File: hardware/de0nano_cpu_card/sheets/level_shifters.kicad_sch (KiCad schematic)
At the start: 10 parts, among them J2 EXP_HEADER_2x11, U1 SN74LVC8T245, U2 SN74LVC8T245, U3 SN74LVC8T245, U4 SN74LVC8T245, U5 SN74LVC8T245, U6 SN74LVC8T245

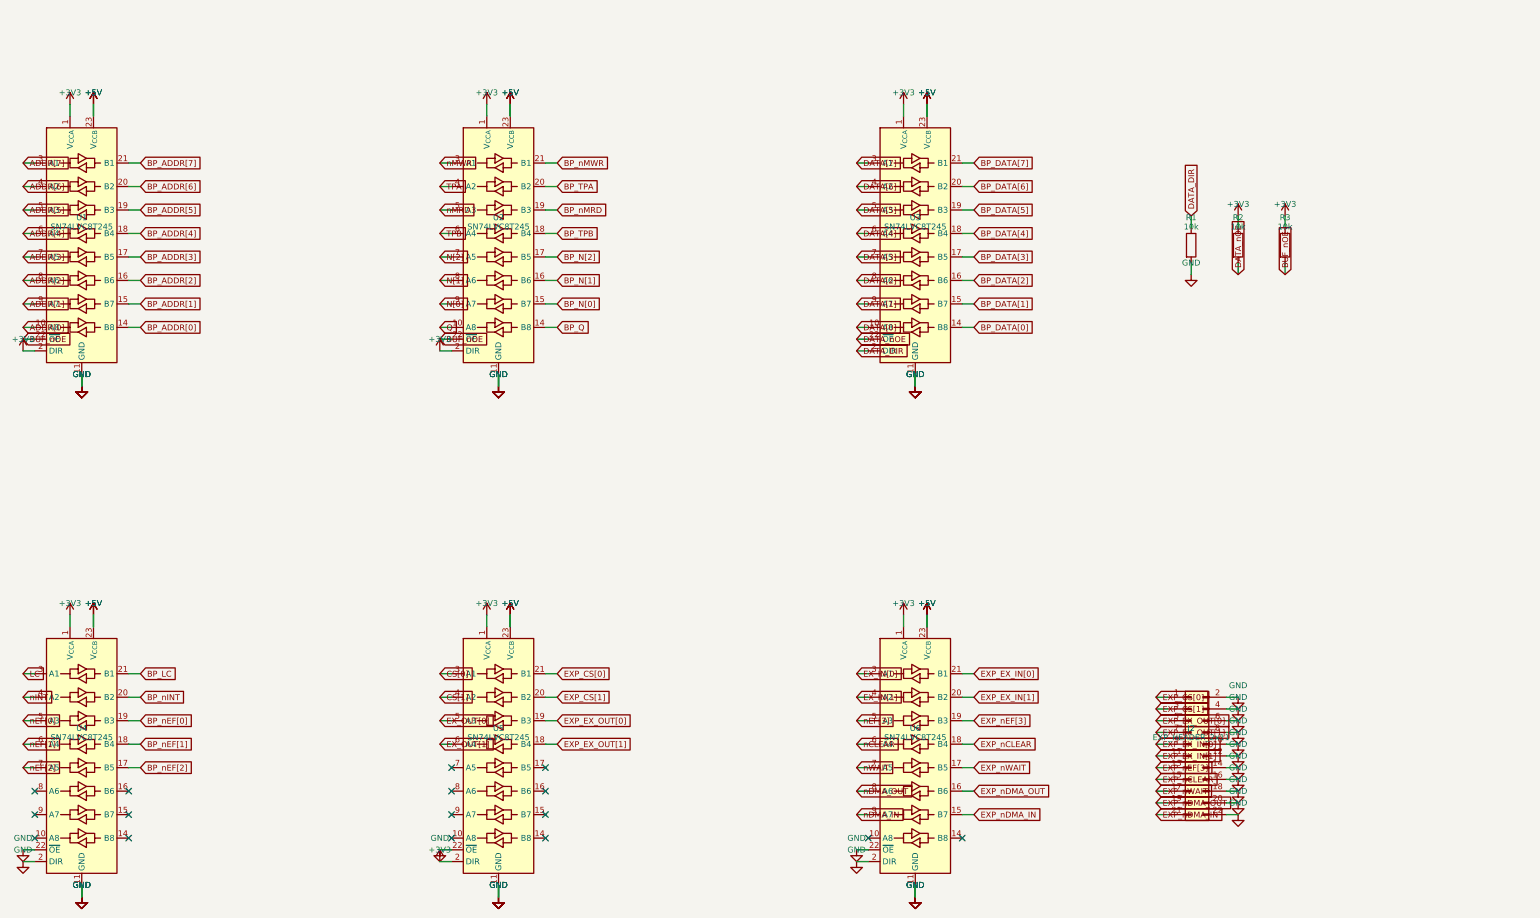
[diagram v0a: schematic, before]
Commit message: Add pull-ups/ties on spare channels and series resistors, per GUI review
The user reviewed the schematics in the KiCad GUI and manually
rearranged component layout on several sheets -- so these fixes are
applied as surgical patches to the current saved files (new
tools/patch_*.py scripts) rather than via the usual build_*.py
regeneration, which would have discarded that layout work. See the new
"don't just re-run build_*.py" section in tools/README.md for the
workflow this establishes going forward.

Electrical changes (level_shifters.kicad_sch):
- 10k pull-up to +5V on all 7 EXP_* future-expansion header input nets
- U4 (backplane IN chip) spare B-side channels (pins 14/15/16): pulled
  out of no_connect, 10k pull-up to +5V each
- U6 (future-expansion IN chip) spare B-side channel (pin 14): pulled
  out of no_connect, 10k pull-up to +5V
- U5 (future-expansion OUT chip) spare A-side channels (pins 7/8/9/10):
  pulled out of no_connect, hard-tied to GND (unused transceiver
  inputs, no resistor needed)

Electrical changes (fpga_header.kicad_sch):
- 10 ohm series resistors on TPA/TPB/nMRD/nMWR at the FPGA end, per
  backplane_notes.md's signal-integrity note (originally suggested
  33-47 ohm; user chose 10 ohm)

sch erc on the full hierarchy: 0 errors. New warnings are the expected
ones (pin_to_pin on the GND hard-ties -- that's what a hard tie looks
like to ERC). pcb drc: 0 violations.

Also includes the project files as resaved by KiCad 10's GUI during
the user's review pass (sheet_instances/project-settings expansion,
plus the user's own layout rearrangement on all 7 sheets), and
gitignores the .history/ directory KiCad 10's local version-history
feature creates.

Co-Authored-By: Claude Sonnet 5 <noreply@anthropic.com>
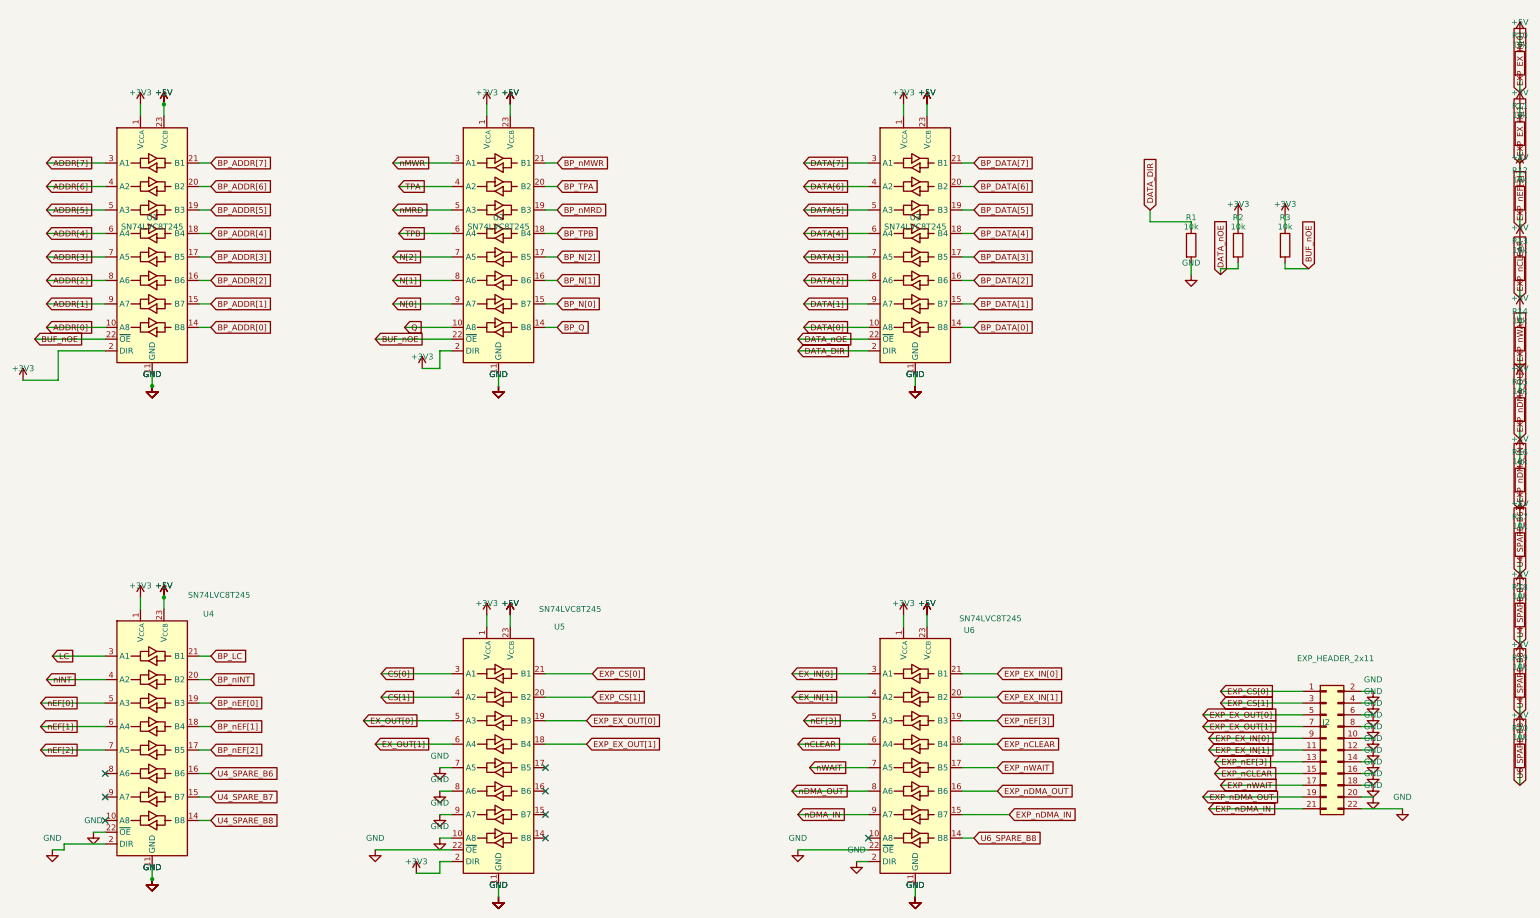
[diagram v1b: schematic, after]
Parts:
- added R10, R11, R12, R13, R14, R15, R16, R17, R18, R19, R20: 10k, Resistor_SMD:R_0603_1608Metric, symbol Device:R
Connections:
- net +5V: now also R10.1, R11.1, R12.1, R13.1, R14.1, R15.1, R16.1, R17.1, R18.1, R19.1, R20.1
- net EXP_EX_IN[0]: now also R10.2
- net EXP_EX_IN[1]: now also R11.2
- net EXP_nCLEAR: now also R13.2
- net EXP_nDMA_IN: now also R16.2
- net EXP_nDMA_OUT: now also R15.2
- net EXP_nEF[3]: now also R12.2
- net EXP_nWAIT: now also R14.2
- net GND: now also U5.10 (A8), U5.7 (A5), U5.8 (A6), U5.9 (A7)
- net U4_SPARE_B8: now reaches U4.14 (B8)
- net U4_SPARE_B8: now also R19.2
- net U4_SPARE_B7: now reaches U4.15 (B7)
- net U4_SPARE_B7: now also R18.2
- net U4_SPARE_B6: now reaches U4.16 (B6)
- net U4_SPARE_B6: now also R17.2
- net U6_SPARE_B8: now reaches U6.14 (B8)
- net U6_SPARE_B8: now also R20.2
- no-connect marks 16 -> 8
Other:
- moved on the sheet: J2, U1, U4
